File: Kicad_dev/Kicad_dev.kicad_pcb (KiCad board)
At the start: 2 copper layers, 31 parts, among them J1 Conn_01x02_Pin, J2 Conn_01x02_Pin, J3 Conn_01x02_Pin, J4 530470510_Picoblade, J5 Connecteur_SMA, J6 BNC, Q1 IRF540N, SW1 RotaryEncoder_Switch, SW2 RotaryEncoder_Switch, U11 MAX-8Q, U12 COM-09032, U2 COM-09032, U3 74HC04, U4 L293D, U5 LM358, U6 PC817_SMD, U7 PC817_THT, U8 NEO-M8Q

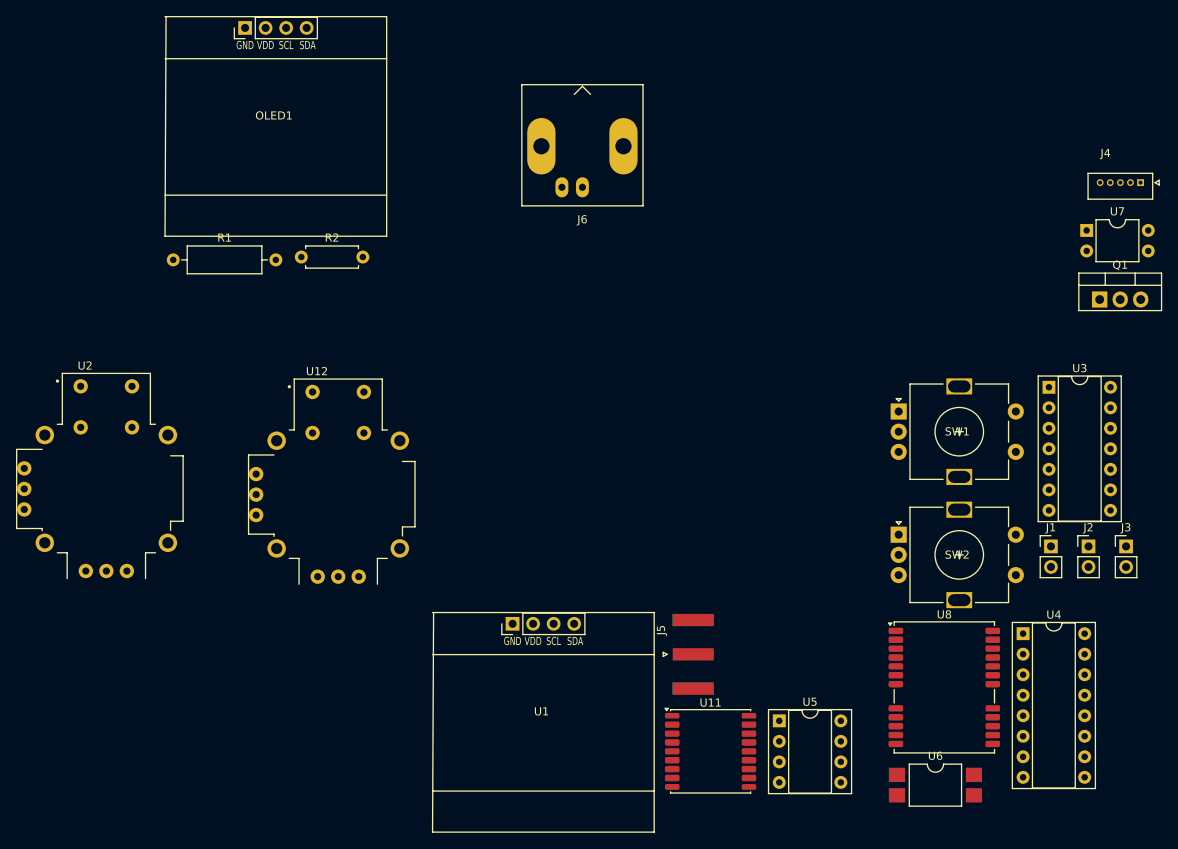
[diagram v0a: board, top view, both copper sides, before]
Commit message: Add repo of lib Kicad before analyzing...
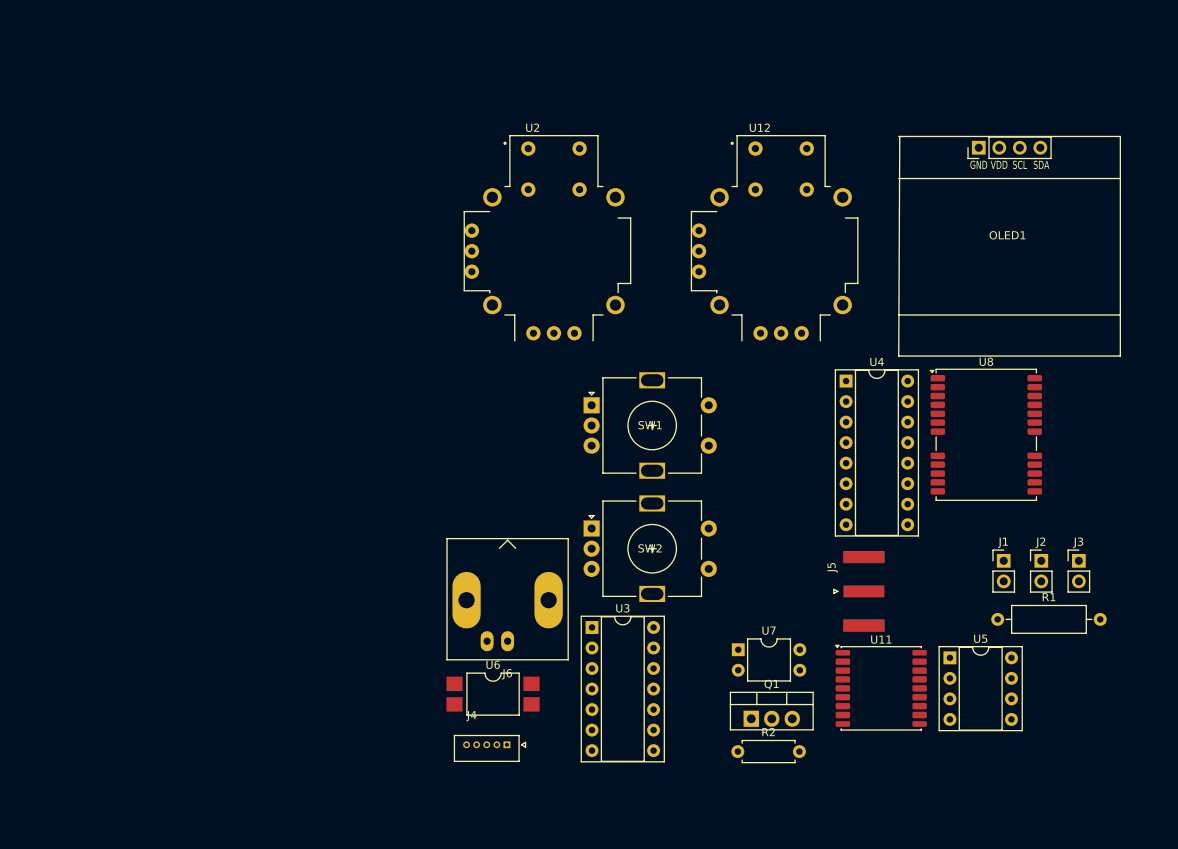
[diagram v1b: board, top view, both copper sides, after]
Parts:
- removed U1: ~, CREPP_Screens:SSD1306_OLED_Display(128x64)
- moved R1 111.3 mm to (151.2, 111.9)
- moved J4 104.8 mm to (90.5, 127.4)
- moved OLED1 92.0 mm to (152.7, 53.5)
- moved R2 81.6 mm to (119.1, 128.3)
- moved V1 71.3 mm to (155.7, 116.4)
- moved U7 67.5 mm to (119.1, 115.7)
- moved Q1 67.5 mm to (120.7, 124.2)
- moved U3 63.9 mm to (101.0, 112.9)
- moved U2 62.7 mm to (96.3, 66.3)
- moved U12 62.6 mm to (124.4, 66.3)
- moved J6 56.9 mm to (90.6, 114.6)
- moved U6 55.9 mm to (88.8, 121.2)
- moved JP1 51.9 mm to (156.8, 127.8)
- moved JP2 51.9 mm to (160.4, 127.8)
- moved JP3 51.9 mm to (164.1, 127.8)
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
